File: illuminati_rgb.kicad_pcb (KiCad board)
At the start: 2 copper layers, 69 x 42 mm, 48 parts, among them IC1 TPS564247DRLR, IC2 SPH0645LM4H-1-8, J1 Conn_02x03_Odd_Even, J2 Conn_01x04, J3 Conn_01x02, J6 Conn_01x02, J7 Conn_01x04, J8 Conn_01x04, Q1 C351406, Q2 C351406, Q3 C351406, Q4 C351406, Q5 C351406, Q6 C351406, Q7 C351406, Q8 C351406, Q9 C351406, SW1 SW_SPST, U1 ESP32-WROOM-32

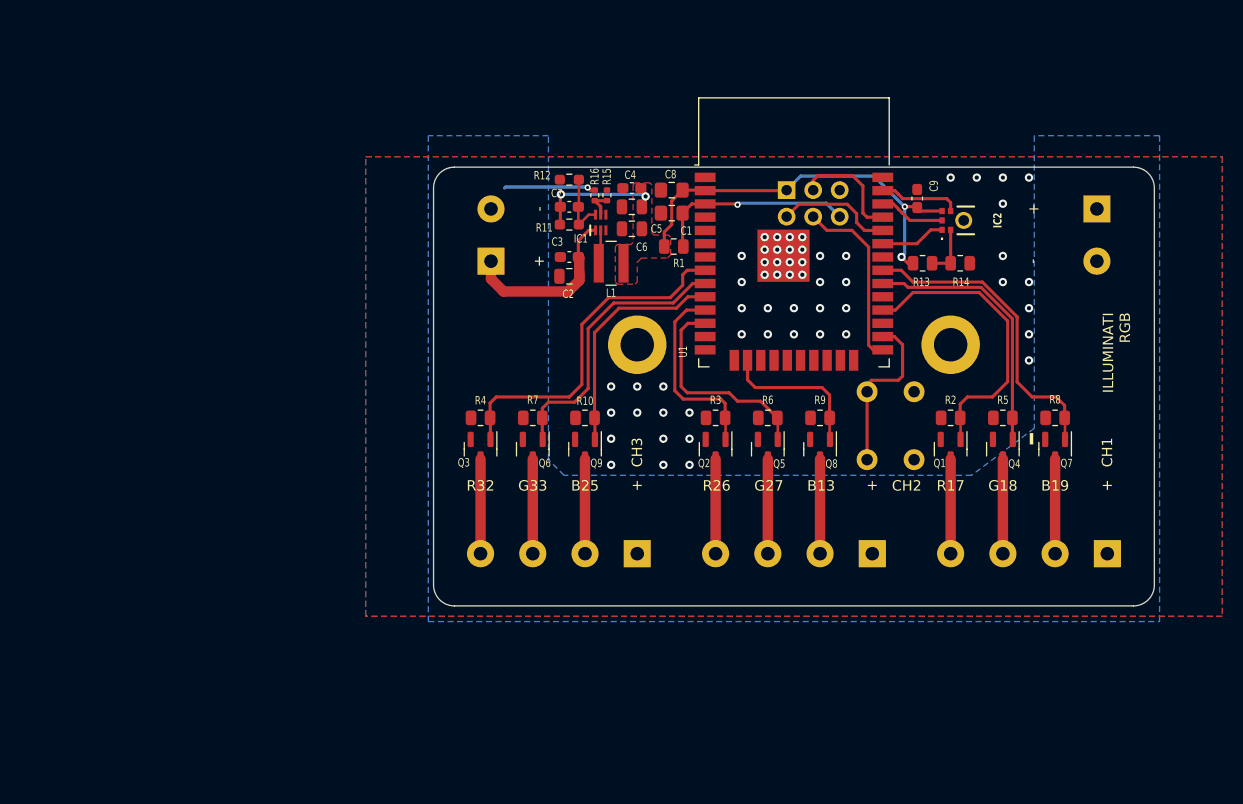
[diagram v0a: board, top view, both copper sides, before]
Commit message: v2 board
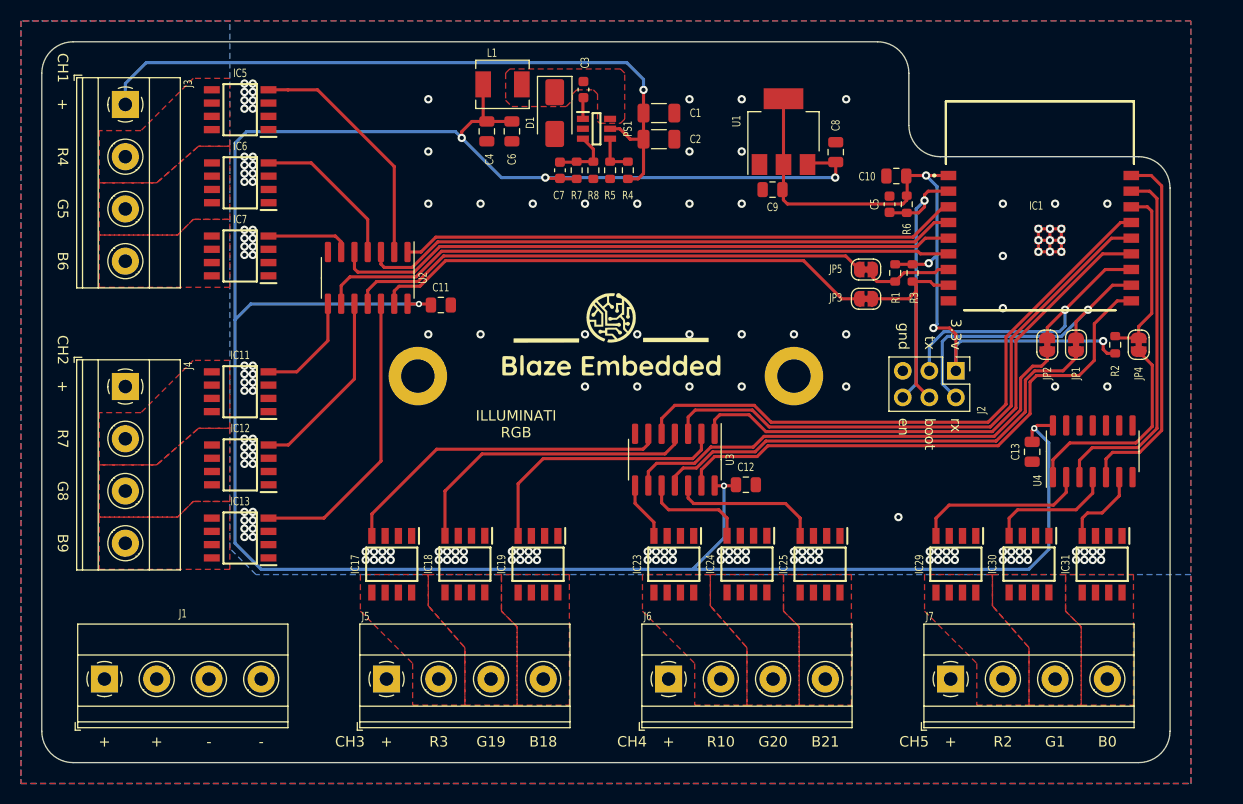
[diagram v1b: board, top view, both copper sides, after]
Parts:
- removed the C5 at (139.5, 87.8)
- removed IC2: SPH0645LM4H-1-8, SamacSys_Parts:SPH0645LM4H18
- removed the J2 at (185.0, 121.0)
- removed J8: Conn_01x04, TerminalBlock_Phoenix:TerminalBlock_Phoenix_MKDS-1,5-4_1x04_P5.00mm_Horizontal
- removed Q1, Q2, Q3, Q4, Q5, Q6, Q7, Q8, Q9: C351406, Package_TO_SOT_SMD:SOT-23
- removed R10, R9: 10k, Resistor_SMD:R_0805_2012Metric
- removed R11: 100k, Resistor_SMD:R_0603_1608Metric_Pad0.98x0.95mm_HandSolder
- removed R12: 22k, Resistor_SMD:R_0603_1608Metric_Pad0.98x0.95mm_HandSolder
- removed R13: NC, Resistor_SMD:R_0805_2012Metric
- removed R14: 0R, Resistor_SMD:R_0805_2012Metric
- removed R15: 10k, Resistor_SMD:R_0402_1005Metric
- removed R16: 20k, Resistor_SMD:R_0402_1005Metric
- removed the R6 at (152.5, 108.0)
- removed SW1: SW_SPST, Button_Switch_THT:SW_PUSH_6mm_H5mm
- added C1: 10u/1206, Capacitor_SMD:C_1206_3216Metric, F.Cu at (142.1, 78.8)
- added C11: 22u, Capacitor_SMD:C_0805_2012Metric, F.Cu at (121.2, 97.2)
- added C12: 22u, Capacitor_SMD:C_0805_2012Metric, F.Cu at (150.4, 114.4)
- added C13: 22u, Capacitor_SMD:C_0805_2012Metric, F.Cu at (177.8, 111.2)
- added C8: 22u, Capacitor_SMD:C_0805_2012Metric, F.Cu at (159.0, 82.6)
- added D1: B340A, Diode_SMD:D_SMA, F.Cu at (132.1, 78.8)
- added G***: LOGO, LOGO, B.Cu at (137.5, 108.0)
- added IC11: SI4174DY-T1-GE3, SamacSys_Parts:SOIC127P600X175-8N, F.Cu at (102.0, 105.5)
- added IC12: SI4174DY-T1-GE3, SamacSys_Parts:SOIC127P600X175-8N, F.Cu at (102.0, 112.5)
- added IC13: SI4174DY-T1-GE3, SamacSys_Parts:SOIC127P600X175-8N, F.Cu at (102.0, 119.5)
- added IC17: SI4174DY-T1-GE3, SamacSys_Parts:SOIC127P600X175-8N, F.Cu at (116.5, 122.0)
- added IC18: SI4174DY-T1-GE3, SamacSys_Parts:SOIC127P600X175-8N, F.Cu at (123.5, 122.0)
- added IC19: SI4174DY-T1-GE3, SamacSys_Parts:SOIC127P600X175-8N, F.Cu at (130.5, 122.0)
- added IC23: SI4174DY-T1-GE3, SamacSys_Parts:SOIC127P600X175-8N, F.Cu at (143.5, 122.0)
- added IC24: SI4174DY-T1-GE3, SamacSys_Parts:SOIC127P600X175-8N, F.Cu at (150.5, 122.0)
- added IC25: SI4174DY-T1-GE3, SamacSys_Parts:SOIC127P600X175-8N, F.Cu at (157.5, 122.0)
- added IC29: SI4174DY-T1-GE3, SamacSys_Parts:SOIC127P600X175-8N, F.Cu at (170.5, 122.0)
- added IC30: SI4174DY-T1-GE3, SamacSys_Parts:SOIC127P600X175-8N, F.Cu at (177.5, 122.0)
- added IC31: SI4174DY-T1-GE3, SamacSys_Parts:SOIC127P600X175-8N, F.Cu at (184.5, 122.0)
- added IC5: SI4174DY-T1-GE3, SamacSys_Parts:SOIC127P600X175-8N, F.Cu at (102.0, 78.5)
- added IC6: SI4174DY-T1-GE3, SamacSys_Parts:SOIC127P600X175-8N, F.Cu at (102.0, 85.5)
- added IC7: SI4174DY-T1-GE3, SamacSys_Parts:SOIC127P600X175-8N, F.Cu at (102.0, 92.5)
- added J1: Conn_01x04, TerminalBlock_Phoenix:TerminalBlock_Phoenix_MKDS-1,5-4_1x04_P5.00mm_Horizontal, F.Cu at (89.0, 133.0)
- added J4: Conn_01x04, TerminalBlock_Phoenix:TerminalBlock_Phoenix_MKDS-1,5-4_1x04_P5.00mm_Horizontal, F.Cu at (91.0, 105.0)
- added J5: Conn_01x04, TerminalBlock_Phoenix:TerminalBlock_Phoenix_MKDS-1,5-4_1x04_P5.00mm_Horizontal, F.Cu at (116.0, 133.0)
- added JP1: Jumper_2_Bridged, Jumper:SolderJumper-2_P1.3mm_Bridged_RoundedPad1.0x1.5mm, F.Cu at (182.0, 101.0)
- added JP2: Jumper_2_Bridged, Jumper:SolderJumper-2_P1.3mm_Bridged_RoundedPad1.0x1.5mm, F.Cu at (179.2, 101.0)
- added JP3: Jumper_2_Bridged, Jumper:SolderJumper-2_P1.3mm_Bridged_RoundedPad1.0x1.5mm, F.Cu at (161.9, 96.6)
- added JP4: Jumper_2_Bridged, Jumper:SolderJumper-2_P1.3mm_Bridged_RoundedPad1.0x1.5mm, F.Cu at (188.0, 101.0)
- added JP5: Jumper_2_Bridged, Jumper:SolderJumper-2_P1.3mm_Bridged_RoundedPad1.0x1.5mm, F.Cu at (161.9, 93.8)
- added PS1: AP5100WG-7, SamacSys_Parts:SOT95P285X140-6N, F.Cu at (136.1, 80.3)
- added R1: 10k, Resistor_SMD:R_0603_1608Metric, F.Cu at (164.7, 94.1)
- added U2: 74HC14, Package_SO:SOIC-14_3.9x8.7mm_P1.27mm, F.Cu at (114.2, 94.6)
- added U3: 74HC14, Package_SO:SOIC-14_3.9x8.7mm_P1.27mm, F.Cu at (143.6, 112.0)
- added U4: 74HC14, Package_SO:SOIC-14_3.9x8.7mm_P1.27mm, F.Cu at (183.6, 111.2)
- C10: renamed from C8; value 10u -> 22u; footprint Capacitor_SMD:C_0805_2012Metric_Pad1.18x1.45mm_HandSolder -> Capacitor_SMD:C_0805_2012Metric
- C2: value 22u -> 10u/1206; footprint Capacitor_SMD:C_0805_2012Metric -> Capacitor_SMD:C_1206_3216Metric
- C3: value 100n -> 22n; footprint Capacitor_SMD:C_0603_1608Metric_Pad1.08x0.95mm_HandSolder -> Capacitor_SMD:C_0603_1608Metric
- C4, C9: value 100n -> 22u; footprint Capacitor_SMD:C_0603_1608Metric_Pad1.08x0.95mm_HandSolder -> Capacitor_SMD:C_0805_2012Metric
- C5: renamed from C1; footprint Capacitor_SMD:C_0805_2012Metric_Pad1.18x1.45mm_HandSolder -> Capacitor_SMD:C_0603_1608Metric
- C7: value 56p -> 100p; footprint Capacitor_SMD:C_0603_1608Metric_Pad1.08x0.95mm_HandSolder -> Capacitor_SMD:C_0603_1608Metric
- G***, J7: moved to F.Cu
- IC1: value TPS564247DRLR -> ESP32-C3-WROOM-02-N4; footprint SamacSys_Parts:SOT50P160X60-6N -> SamacSys_Parts:ESP32C3WROOM02N4
- J2: renamed from J1; moved to F.Cu
- J3, J6: value Conn_01x02 -> Conn_01x04; footprint TerminalBlock_Phoenix:TerminalBlock_Phoenix_MKDS-1,5-2_1x02_P5.00mm_Horizontal -> TerminalBlock_Phoenix:TerminalBlock_Phoenix_MKDS-1,5-4_1x04_P5.00mm_Horizontal; moved to F.Cu
- L1: value 1.5u -> 10u/C2921170; footprint Inductor_SMD:L_Wuerth_MAPI-4020 -> Inductor_SMD:L_Chilisin_BMRA00040420
- R2, R3, R4, R7: footprint Resistor_SMD:R_0805_2012Metric -> Resistor_SMD:R_0603_1608Metric
- R5, R8: value 10k -> 2k; footprint Resistor_SMD:R_0805_2012Metric -> Resistor_SMD:R_0603_1608Metric
- R6: renamed from R1; footprint Resistor_SMD:R_0805_2012Metric -> Resistor_SMD:R_0603_1608Metric
- U1: value ESP32-WROOM-32 -> AMS1117-3.3; footprint RF_Module:ESP32-WROOM-32 -> Package_TO_SOT_SMD:SOT-223-3_TabPin2
- moved J6 60.9 mm to (143.0, 133.0), turned to 0 degrees
- moved R8 50.2 mm to (135.8, 84.3), turned to -90 degrees
- moved R5 44.4 mm to (137.4, 84.3), turned to 90 degrees
- moved IC1 43.0 mm to (179.5, 91.0), turned to 0 degrees
- moved J3 38.1 mm to (91.0, 78.0), turned to -90 degrees
- moved R4 27.6 mm to (139.1, 84.3), turned to -90 degrees
- moved R7 24.1 mm to (134.2, 84.3), turned to 90 degrees
- moved J2 23.7 mm to (170.5, 103.5)
- moved R3 23.4 mm to (166.3, 94.1), turned to -90 degrees
- moved R6 22.7 mm to (165.8, 87.5), turned to -90 degrees
- moved C10 21.5 mm to (164.8, 84.8)
- moved H1 21.2 mm to (119.0, 104.0)
- moved C5 20.9 mm to (164.2, 87.5), turned to 90 degrees
- moved L1 20.0 mm to (127.1, 76.1)
- moved G*** 19.0 mm to (137.5, 100.0), turned to 0 degrees
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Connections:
- C3 pad 1: VCC -> Net-(PS1-BST)
- C3 pad 2: GND -> Net-(D1-K)
- C4 pad 1: +3V3 -> +5V
- C6 pad 1: +3V3 -> +5V
- C7 pad 1: +3V3 -> +5V
- C7 pad 2: Net-(IC1-FB) -> /V_FB
- C9 pad 1: GND -> +3V3
- C9 pad 2: +3V3 -> GND
- IC1 pad 1: VCC -> +3V3
- IC1 pad 2: Net-(IC1-SW) -> /esp_en
- IC1 pad 3: GND -> /R1
- IC1 pad 4: GND -> /G1
- IC1 pad 5: Net-(IC1-EN) -> /B1
- IC1 pad 6: Net-(IC1-FB) -> /R2
- J3 pad 2: GND -> /RGB Channel1/OUT_R
- J6 pad 2: GND -> /RGB Channel4/OUT_R
- J7 pad 2: /B2_OUT -> /RGB Channel5/OUT_R
- J7 pad 3: /G2_OUT -> /RGB Channel5/OUT_G
- J7 pad 4: /R2_OUT -> /RGB Channel5/OUT_B
- L1 pad 1: +3V3 -> Net-(D1-K)
- L1 pad 2: Net-(IC1-SW) -> +5V
- R2 pad 1: /R1 -> +3V3
- R2 pad 2: GND -> /gpio2
- R3 pad 1: /R2 -> +3V3
- R3 pad 2: GND -> /boot
- R4 pad 1: /R3 -> Net-(PS1-EN)
- R4 pad 2: GND -> VCC
- R5 pad 1: /G1 -> GND
- R5 pad 2: GND -> Net-(PS1-EN)
- R7 pad 1: /G3 -> +5V
- R7 pad 2: GND -> /V_FB
- R8 pad 1: /B1 -> /V_FB
- U1 pad 3: /esp_en -> +5V
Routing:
- net +5V: track 0.00 -> 242.0 mm, vias 0 -> 6
- net /B4: track 0.00 -> 53.2 mm
- net /R4: track 0.00 -> 46.6 mm
- net /G4: track 0.00 -> 46.4 mm
- net /R2: track 18.7 -> 61.3 mm
- net VCC: track 25.8 -> 67.4 mm
- net /G5: track 0.00 -> 35.1 mm
- net /B5: track 0.00 -> 34.9 mm
- net /B2: track 14.6 -> 48.4 mm
- net /RGB Channel3/R: track 0.00 -> 32.3 mm
- net /G1: track 25.4 -> 57.4 mm
- net /B3: track 22.2 -> 52.9 mm
- net /B1: track 29.7 -> 59.9 mm
- net /G2: track 20.5 -> 50.2 mm
- net /G3: track 26.9 -> 56.2 mm
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- added copper zone on F.Cu, net /RGB Channel1/OUT_B
- added copper zone on F.Cu, net /RGB Channel1/OUT_G
- added copper zone on F.Cu, net /RGB Channel1/OUT_R
- added copper zone on F.Cu, net /RGB Channel2/OUT_B
- added copper zone on F.Cu, net /RGB Channel2/OUT_G
- added copper zone on F.Cu, net /RGB Channel2/OUT_R
- added copper zone on F.Cu, net /RGB Channel3/OUT_B
- added copper zone on F.Cu, net /RGB Channel3/OUT_G
- added copper zone on F.Cu, net /RGB Channel3/OUT_R
- added copper zone on F.Cu, net /RGB Channel4/OUT_B
- added copper zone on F.Cu, net /RGB Channel4/OUT_G
- added copper zone on F.Cu, net /RGB Channel4/OUT_R
- added copper zone on F.Cu, net /RGB Channel5/OUT_B
- added copper zone on F.Cu, net /RGB Channel5/OUT_G
- added copper zone on F.Cu, net /RGB Channel5/OUT_R
- added copper zone on F.Cu, net Net-(D1-K)
- removed copper zone on F.Cu, net +3V3
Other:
- board size 69 x 42 mm -> 108 x 69 mm
- board text added: "3.3v"
- board text added: "B0"
- board text added: "B18"
- board text added: "B21"
- board text added: "B6"
- board text added: "B9"
- board text added: "CH4"
- board text added: "CH5"
- board text added: "G1"
- board text added: "G19"
- board text added: "G20"
- board text added: "G5"
- board text added: "G8"
- board text added: "R10"
- board text added: "R2"
- board text added: "R3"
- board text added: "R4"
- board text added: "R7"
- board text added: "boot"
- board text added: "en"
- board text added: "gnd"
- board text added: "rx"
- board text added: "tx"
- board text removed: "B13"
- board text removed: "B19"
- board text removed: "B25"
- board text removed: "G18"
- board text removed: "G27"
- board text removed: "G33"
- board text removed: "R17"
- board text removed: "R26"
- board text removed: "R32"
